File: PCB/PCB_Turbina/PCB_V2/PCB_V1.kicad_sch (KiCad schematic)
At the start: 14 parts, among them J1 BATT_11.1V, J2 Conn_01x07, J3 ENODER_LEFT, J4 ENODER_RIGH, J5 BATT_7.4V, J6 JST-7.7V, J7 TURBINE_POWER, J8 TURBINE_PWM, J9 Modulo de arranque, SW1 Switch, U1 WeMos_S2_mini, U2 MOTOR_LEFT, U3 MOTOR_RIGH, U4 LM1117T-3.3

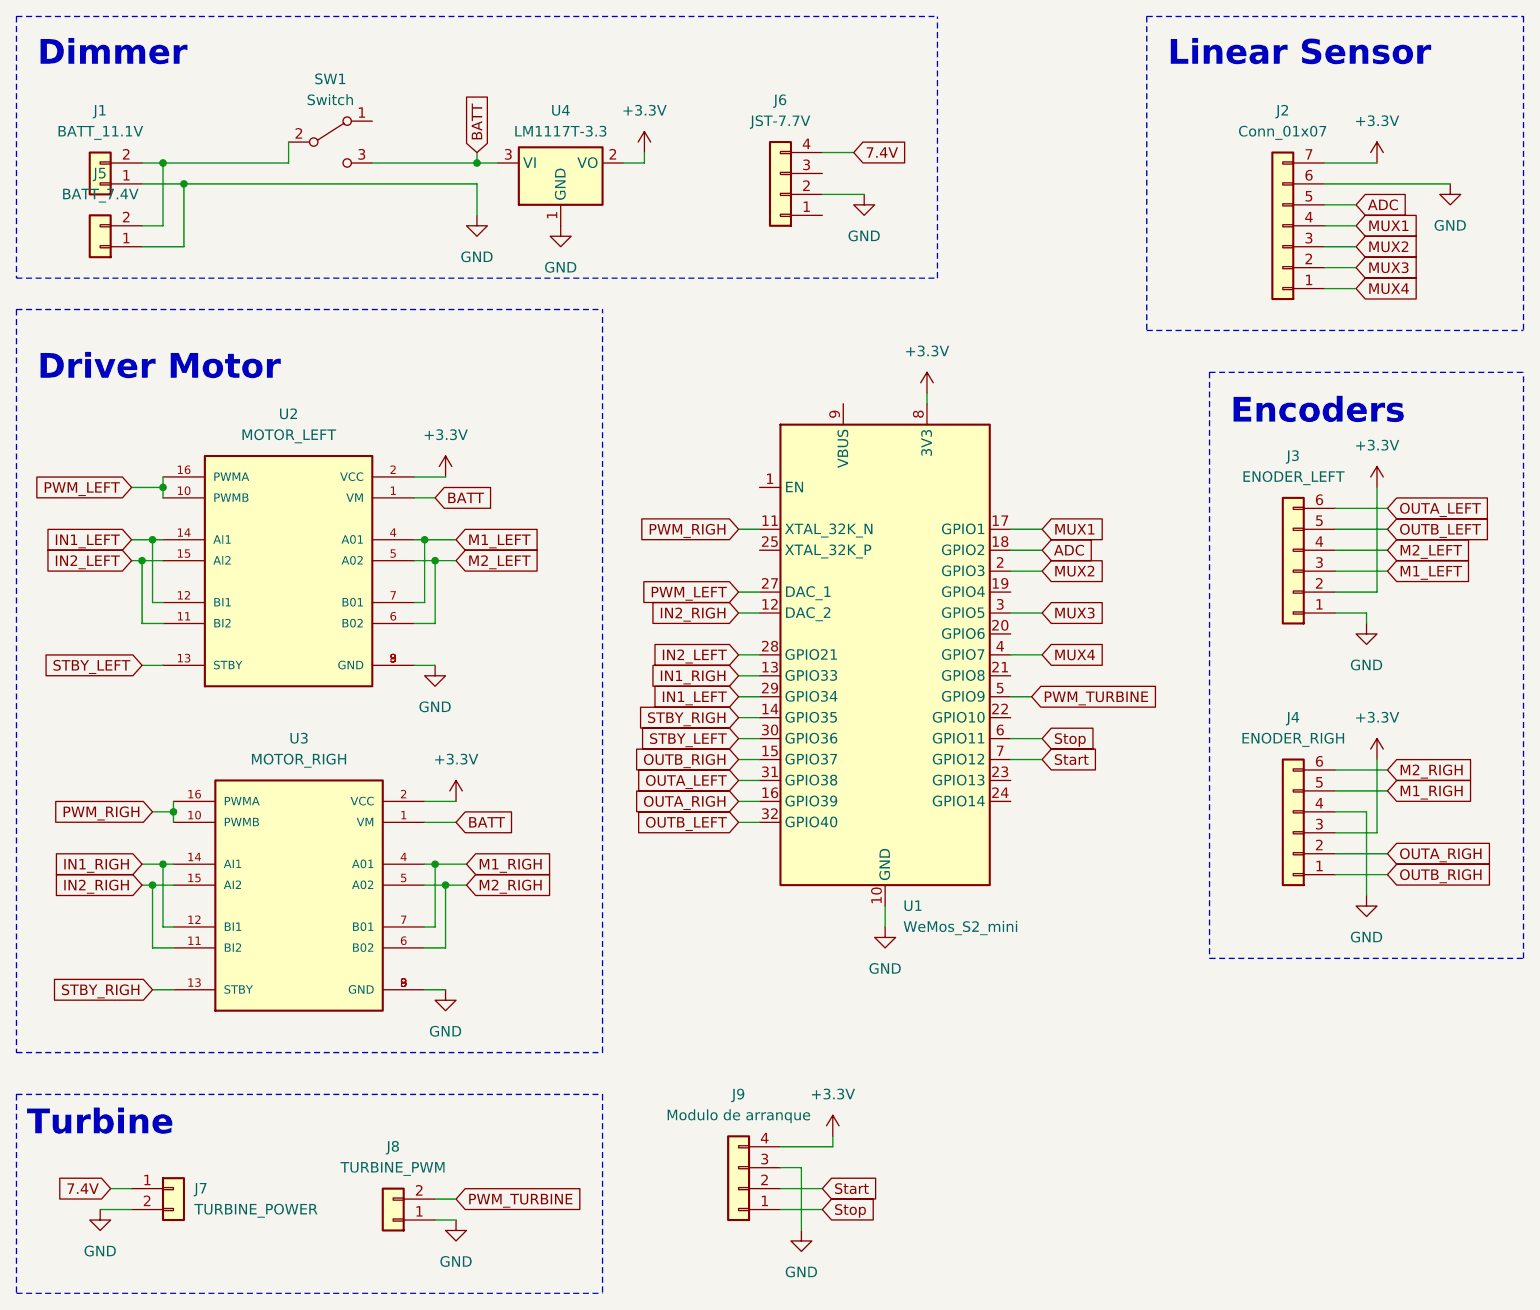
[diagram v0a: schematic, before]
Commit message: PCB_V3
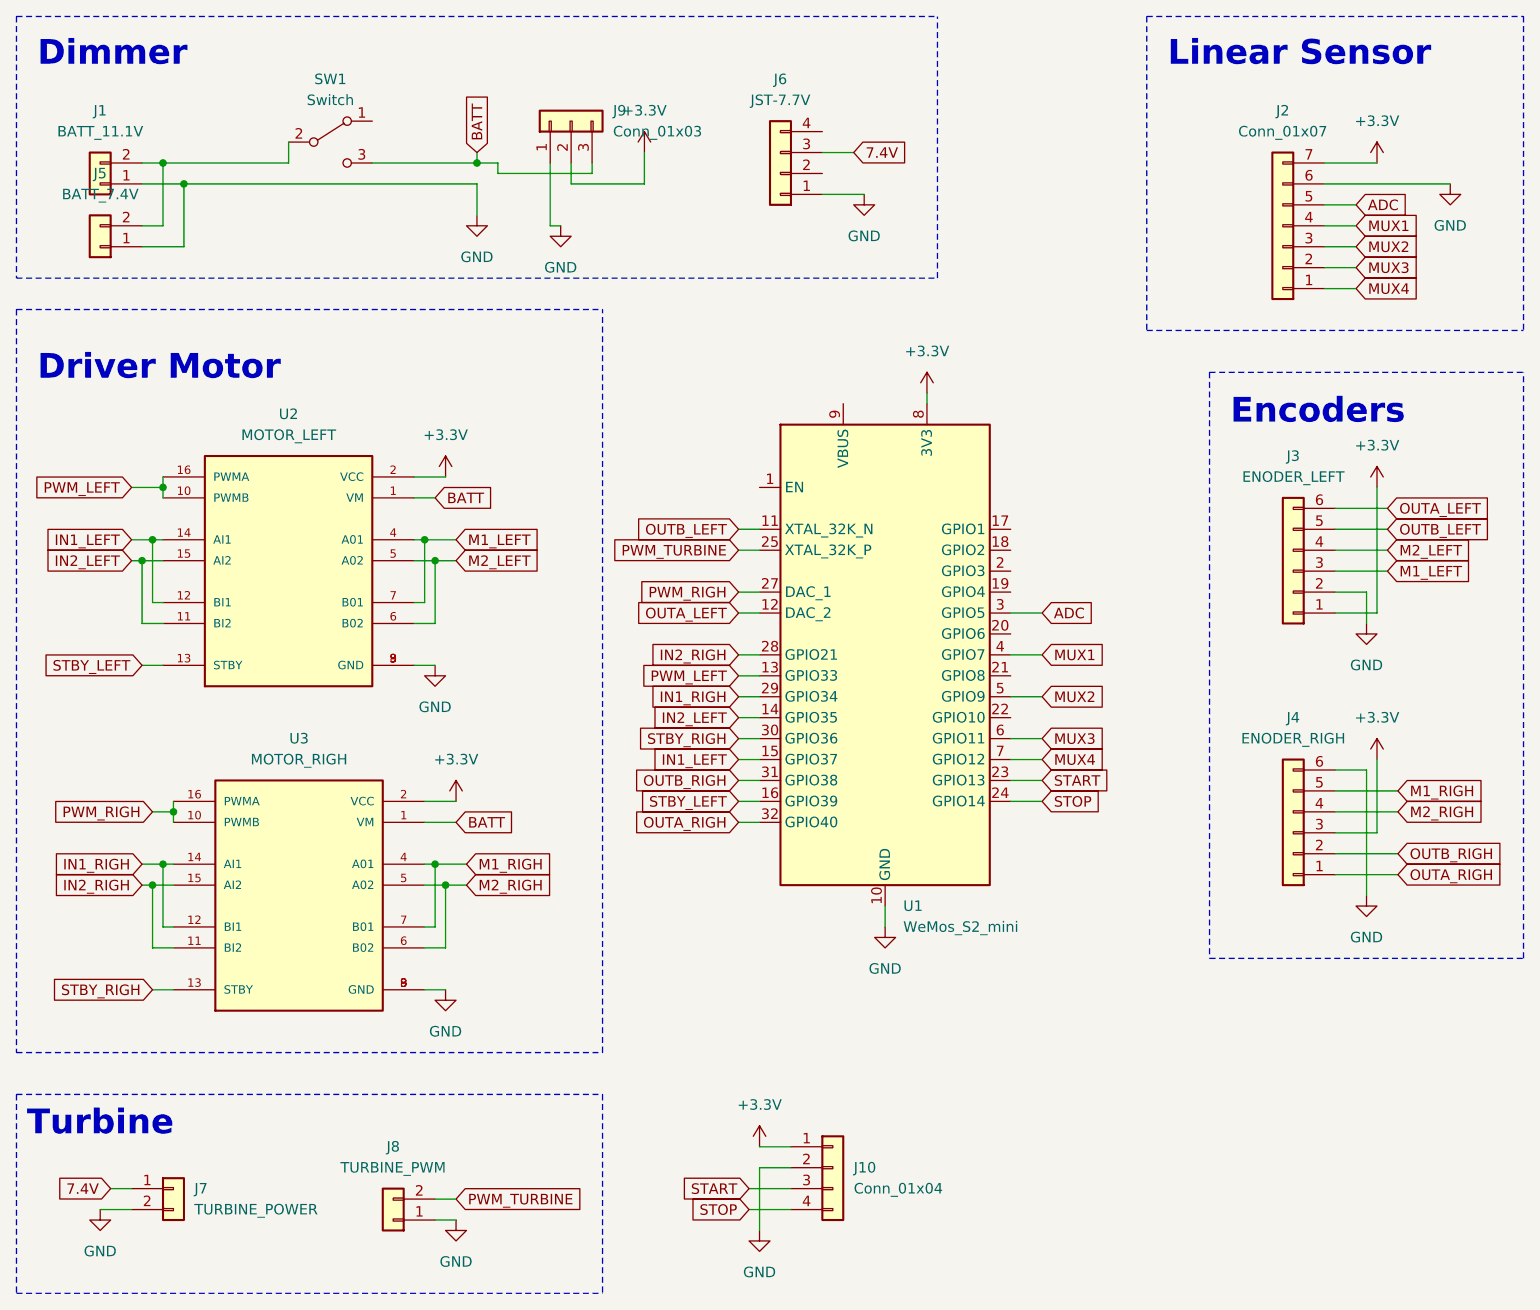
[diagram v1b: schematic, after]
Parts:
- removed J9: Modulo de arranque, Connector_PinHeader_2.54mm:PinHeader_1x04_P2.54mm_Vertical, symbol Connector_Generic:Conn_01x04
- removed U4: LM1117T-3.3, Package_TO_SOT_THT:TO-220-3_Horizontal_TabDown, symbol Regulator_Linear:LM1117T-3.3
- added J10: Conn_01x04, Connector_PinHeader_2.54mm:PinHeader_1x04_P2.54mm_Vertical, symbol Connector_Generic:Conn_01x04
- added J9: Conn_01x03, Connector_PinHeader_2.54mm:PinHeader_1x03_P2.54mm_Vertical, symbol Connector_Generic:Conn_01x03
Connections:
- net Start is gone; now on net MUX4: U1.7 (GPIO12)
- net Stop is gone; now on net MUX3: U1.6 (GPIO11)
- net +3.3V: now also J3.1 (Pin_1), J10.1 (Pin_1), J9.2 (Pin_2); no longer J3.2 (Pin_2)
- net 7.4V: now also J6.3 (Pin_3); no longer J6.4 (Pin_4)
- net ADC: now also U1.3 (GPIO5); no longer U1.18 (GPIO2)
- net BATT: now also J9.3 (Pin_3)
- net GND: now also J3.2 (Pin_2), J4.6 (Pin_6), J6.1 (Pin_1), J10.2 (Pin_2), J9.1 (Pin_1); no longer J3.1 (Pin_1), J4.4 (Pin_4), J6.2 (Pin_2)
- net IN1_LEFT: now also U1.15 (GPIO37); no longer U1.29 (GPIO34)
- net IN1_RIGH: now also U1.29 (GPIO34); no longer U1.13 (GPIO33)
- net IN2_LEFT: now also U1.14 (GPIO35); no longer U1.28 (GPIO21)
- net IN2_RIGH: now also U1.28 (GPIO21); no longer U1.12 (DAC_2)
- net M2_RIGH: now also J4.4 (Pin_4); no longer J4.6 (Pin_6)
- net MUX1: now also U1.4 (GPIO7); no longer U1.17 (GPIO1)
- net MUX2: now also U1.5 (GPIO9); no longer U1.2 (GPIO3)
- net MUX3: no longer U1.3 (GPIO5)
- net MUX4: no longer U1.4 (GPIO7)
- net OUTA_LEFT: now also U1.12 (DAC_2); no longer U1.31 (GPIO38)
- net OUTA_RIGH: now also J4.1 (Pin_1), U1.32 (GPIO40); no longer J4.2 (Pin_2), U1.16 (GPIO39)
- net OUTB_LEFT: now also U1.11 (XTAL_32K_N); no longer U1.32 (GPIO40)
- net OUTB_RIGH: now also J4.2 (Pin_2), U1.31 (GPIO38); no longer J4.1 (Pin_1), U1.15 (GPIO37)
- net PWM_LEFT: now also U1.13 (GPIO33); no longer U1.27 (DAC_1)
- net PWM_RIGH: now also U1.27 (DAC_1); no longer U1.11 (XTAL_32K_N)
- net PWM_TURBINE: now also U1.25 (XTAL_32K_P); no longer U1.5 (GPIO9)
- net STBY_LEFT: now also U1.16 (GPIO39); no longer U1.30 (GPIO36)
- net STBY_RIGH: now also U1.30 (GPIO36); no longer U1.14 (GPIO35)
- net START: now reaches U1.23 (GPIO13)
- net START: now also J10.3 (Pin_3)
- net STOP: now reaches U1.24 (GPIO14)
- net STOP: now also J10.4 (Pin_4)
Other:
- moved on the sheet: J6
